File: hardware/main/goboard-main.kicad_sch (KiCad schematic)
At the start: 15 parts, among them J1 USB_C_Receptacle_USB2.0, J2 Conn_02x05_Top_Bottom, J3 Conn_01x01, J4 Conn_01x05, SW11 SW_Push, SW30 SW_DP3T

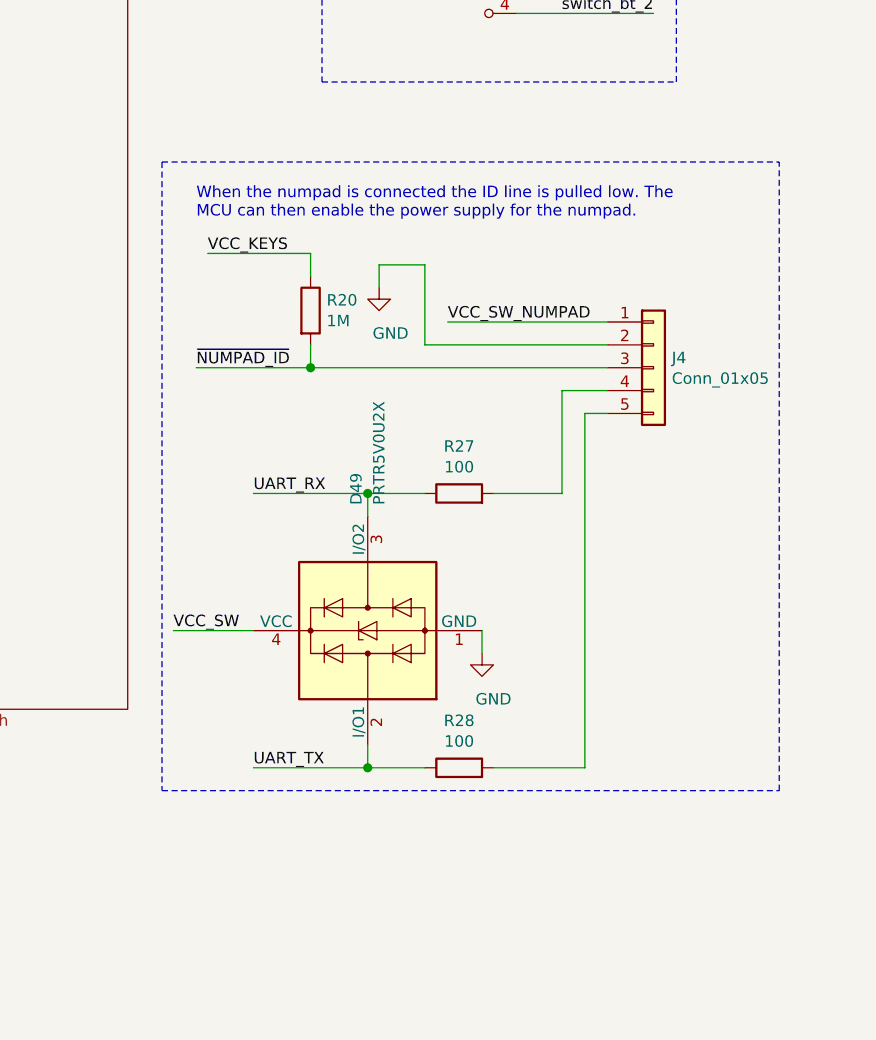
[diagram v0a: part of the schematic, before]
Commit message: WIP: Design of PCB
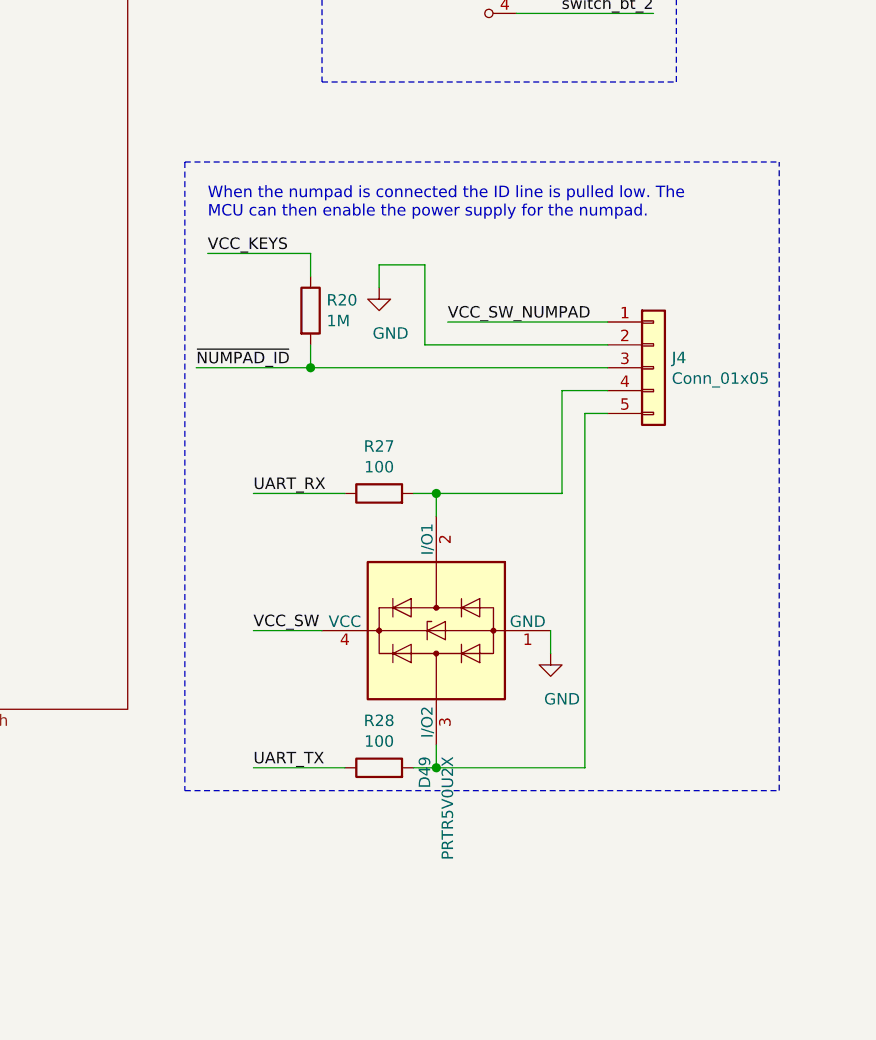
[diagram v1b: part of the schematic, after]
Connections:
- net UART_RX: no longer D49.3 (I/O2)
- net UART_TX: no longer D49.2 (I/O1)
- net at J4.4 (Pin_4), R27.2: now also D49.2 (I/O1)
- net at J4.5 (Pin_5), R28.2: now also D49.3 (I/O2)
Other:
- moved on the sheet: D49, R27, R28
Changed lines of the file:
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@@
   (junction (at 80.01 91.44) (diameter 1.016) (color 0 0 0 0))
   (junction (at 232.41 109.22) (diameter 1.016) (color 0 0 0 0))
-  (junction (at 238.76 123.19) (diameter 1.016) (color 0 0 0 0))
-  (junction (at 238.76 153.67) (diameter 1.016) (color 0 0 0 0))
+  (junction (at 246.38 123.19) (diameter 1.016) (color 0 0 0 0))
+  (junction (at 246.38 153.67) (diameter 1.016) (color 0 0 0 0))
   (no_connect (at 33.02 165.1))
   (no_connect (at 33.02 170.18))
@@
     (stroke (width 0) (type solid) (color 0 0 0 0))
   )
-  (wire (pts (xy 217.17 138.43) (xy 226.06 138.43))
-    (stroke (width 0) (type solid) (color 0 0 0 0))
-  )
   (wire (pts (xy 219.71 109.22) (xy 232.41 109.22))
     (stroke (width 0) (type solid) (color 0 0 0 0))
@@
     (stroke (width 0) (type solid) (color 0 0 0 0))
   )
-  (wire (pts (xy 226.06 123.19) (xy 238.76 123.19))
-    (stroke (width 0) (type solid) (color 0 0 0 0))
-  )
-  (wire (pts (xy 226.06 153.67) (xy 238.76 153.67))
+  (wire (pts (xy 226.06 123.19) (xy 236.22 123.19))
+    (stroke (width 0) (type solid) (color 0 0 0 0))
+  )
+  (wire (pts (xy 226.06 138.43) (xy 233.68 138.43))
+    (stroke (width 0) (type solid) (color 0 0 0 0))
+  )
+  (wire (pts (xy 226.06 153.67) (xy 236.22 153.67))
     (stroke (width 0) (type solid) (color 0 0 0 0))
   )
@@
     (stroke (width 0) (type solid) (color 0 0 0 0))
   )
-  (wire (pts (xy 238.76 123.19) (xy 238.76 125.73))
-    (stroke (width 0) (type solid) (color 0 0 0 0))
-  )
-  (wire (pts (xy 238.76 123.19) (xy 245.11 123.19))
-    (stroke (width 0) (type solid) (color 0 0 0 0))
-  )
-  (wire (pts (xy 238.76 151.13) (xy 238.76 153.67))
-    (stroke (width 0) (type solid) (color 0 0 0 0))
-  )
-  (wire (pts (xy 238.76 153.67) (xy 245.11 153.67))
-    (stroke (width 0) (type solid) (color 0 0 0 0))
-  )
   (wire (pts (xy 240.03 97.79) (xy 240.03 100.33))
     (stroke (width 0) (type solid) (color 0 0 0 0))
@@
     (stroke (width 0) (type solid) (color 0 0 0 0))
   )
+  (wire (pts (xy 243.84 123.19) (xy 246.38 123.19))
+    (stroke (width 0) (type solid) (color 0 0 0 0))
+  )
+  (wire (pts (xy 243.84 153.67) (xy 246.38 153.67))
+    (stroke (width 0) (type solid) (color 0 0 0 0))
+  )
   (wire (pts (xy 245.11 97.79) (xy 245.11 106.68))
     (stroke (width 0) (type solid) (color 0 0 0 0))
@@
     (stroke (width 0) (type solid) (color 0 0 0 0))
   )
+  (wire (pts (xy 246.38 123.19) (xy 246.38 125.73))
+    (stroke (width 0) (type solid) (color 0 0 0 0))
+  )
+  (wire (pts (xy 246.38 123.19) (xy 260.35 123.19))
+    (stroke (width 0) (type solid) (color 0 0 0 0))
+  )
+  (wire (pts (xy 246.38 151.13) (xy 246.38 153.67))
+    (stroke (width 0) (type solid) (color 0 0 0 0))
+  )
+  (wire (pts (xy 246.38 153.67) (xy 262.89 153.67))
+    (stroke (width 0) (type solid) (color 0 0 0 0))
+  )
   (wire (pts (xy 247.65 104.14) (xy 265.43 104.14))
     (stroke (width 0) (type solid) (color 0 0 0 0))
   )
-  (wire (pts (xy 251.46 138.43) (xy 251.46 140.97))
-    (stroke (width 0) (type solid) (color 0 0 0 0))
-  )
-  (wire (pts (xy 252.73 123.19) (xy 260.35 123.19))
-    (stroke (width 0) (type solid) (color 0 0 0 0))
-  )
   (wire (pts (xy 255.27 67.31) (xy 270.51 67.31))
     (stroke (width 0) (type solid) (color 0 0 0 0))
@@
     (stroke (width 0) (type solid) (color 0 0 0 0))
   )
+  (wire (pts (xy 259.08 138.43) (xy 259.08 140.97))
+    (stroke (width 0) (type solid) (color 0 0 0 0))
+  )
   (wire (pts (xy 260.35 111.76) (xy 265.43 111.76))
     (stroke (width 0) (type solid) (color 0 0 0 0))
@@
     (stroke (width 0) (type solid) (color 0 0 0 0))
   )
-  (wire (pts (xy 262.89 153.67) (xy 252.73 153.67))
-    (stroke (width 0) (type solid) (color 0 0 0 0))
-  )
   (wire (pts (xy 265.43 114.3) (xy 262.89 114.3))
     (stroke (width 0) (type solid) (color 0 0 0 0))
   )
-  (polyline (pts (xy 215.9 86.36) (xy 215.9 156.21))
+  (polyline (pts (xy 218.44 86.36) (xy 218.44 156.21))
     (stroke (width 0) (type dash) (color 0 0 0 0))
   )
-  (polyline (pts (xy 215.9 86.36) (xy 284.48 86.36))
+  (polyline (pts (xy 218.44 86.36) (xy 284.48 86.36))
     (stroke (width 0) (type dash) (color 0 0 0 0))
   )
-  (polyline (pts (xy 215.9 156.21) (xy 284.48 156.21))
+  (polyline (pts (xy 218.44 156.21) (xy 284.48 156.21))
     (stroke (width 0) (type dash) (color 0 0 0 0))
   )
@@
   )
   (text "When the numpad is connected the ID line is pulled low. The\nMCU can then enable the power supply for the numpad."
-    (at 219.71 92.71 0)
+    (at 220.98 92.71 0)
     (effects (font (size 1.27 1.27)) (justify left bottom))
   )
@@
     (effects (font (size 1.27 1.27)) (justify right bottom))
   )
-  (label "VCC_SW" (at 217.17 138.43 0)
-    (effects (font (size 1.27 1.27)) (justify left bottom))
-  )
   (label "~NUMPAD_ID" (at 219.71 109.22 0)
     (effects (font (size 1.27 1.27)) (justify left bottom))
@@
   )
   (label "UART_RX" (at 226.06 123.19 0)
+    (effects (font (size 1.27 1.27)) (justify left bottom))
+  )
+  (label "VCC_SW" (at 226.06 138.43 0)
     (effects (font (size 1.27 1.27)) (justify left bottom))
   )
@@
     )
   )
-  (symbol (lib_id "power:GND") (at 251.46 140.97 0) (unit 1)
-    (in_bom yes) (on_board yes)
-    (property "Reference" "#PWR0123" (id 0) (at 251.46 147.32 0)
-      (effects (font (size 1.27 1.27)) hide)
-    )
-    (property "Value" "GND" (id 1) (at 252.73 146.05 0))
-    (property "Footprint" "" (id 2) (at 251.46 140.97 0)
-      (effects (font (size 1.27 1.27)) hide)
-    )
-    (property "Datasheet" "" (id 3) (at 251.46 140.97 0)
+  (symbol (lib_id "power:GND") (at 259.08 140.97 0) (unit 1)
+    (in_bom yes) (on_board yes)
+    (property "Reference" "#PWR0123" (id 0) (at 259.08 147.32 0)
+      (effects (font (size 1.27 1.27)) hide)
+    )
+    (property "Value" "GND" (id 1) (at 260.35 146.05 0))
+    (property "Footprint" "" (id 2) (at 259.08 140.97 0)
+      (effects (font (size 1.27 1.27)) hide)
+    )
+    (property "Datasheet" "" (id 3) (at 259.08 140.97 0)
       (effects (font (size 1.27 1.27)) hide)
     )
@@
     )
   )
-  (symbol (lib_id "Device:R") (at 248.92 123.19 90) (unit 1)
-    (in_bom yes) (on_board yes)
-    (property "Reference" "R27" (id 0) (at 248.92 117.9638 90))
-    (property "Value" "100" (id 1) (at 248.92 120.2625 90))
-    (property "Footprint" "Resistor_SMD:R_0603_1608Metric_Pad0.98x0.95mm_HandSolder" (id 2) (at 248.92 124.968 90)
-      (effects (font (size 1.27 1.27)) hide)
-    )
-    (property "Datasheet" "~" (id 3) (at 248.92 123.19 0)
-      (effects (font (size 1.27 1.27)) hide)
-    )
-  )
-  (symbol (lib_id "Device:R") (at 248.92 153.67 90) (unit 1)
-    (in_bom yes) (on_board yes)
-    (property "Reference" "R28" (id 0) (at 248.92 148.4438 90))
-    (property "Value" "100" (id 1) (at 248.92 150.7425 90))
-    (property "Footprint" "Resistor_SMD:R_0603_1608Metric_Pad0.98x0.95mm_HandSolder" (id 2) (at 248.92 155.448 90)
-      (effects (font (size 1.27 1.27)) hide)
-    )
-    (property "Datasheet" "~" (id 3) (at 248.92 153.67 0)
+  (symbol (lib_id "Device:R") (at 240.03 123.19 90) (unit 1)
+    (in_bom yes) (on_board yes)
+    (property "Reference" "R27" (id 0) (at 240.03 117.9638 90))
+    (property "Value" "100" (id 1) (at 240.03 120.2625 90))
+    (property "Footprint" "Resistor_SMD:R_0603_1608Metric_Pad0.98x0.95mm_HandSolder" (id 2) (at 240.03 124.968 90)
+      (effects (font (size 1.27 1.27)) hide)
+    )
+    (property "Datasheet" "~" (id 3) (at 240.03 123.19 0)
+      (effects (font (size 1.27 1.27)) hide)
+    )
+  )
+  (symbol (lib_id "Device:R") (at 240.03 153.67 90) (unit 1)
+    (in_bom yes) (on_board yes)
+    (property "Reference" "R28" (id 0) (at 240.03 148.4438 90))
+    (property "Value" "100" (id 1) (at 240.03 150.7425 90))
+    (property "Footprint" "Resistor_SMD:R_0603_1608Metric_Pad0.98x0.95mm_HandSolder" (id 2) (at 240.03 155.448 90)
+      (effects (font (size 1.27 1.27)) hide)
+    )
+    (property "Datasheet" "~" (id 3) (at 240.03 153.67 0)
       (effects (font (size 1.27 1.27)) hide)
     )
@@
     )
   )
-  (symbol (lib_id "Power_Protection:PRTR5V0U2X") (at 238.76 138.43 90) (unit 1)
-    (in_bom yes) (on_board yes)
-    (property "Reference" "D49" (id 0) (at 237.49 124.46 0)
-      (effects (font (size 1.27 1.27)) (justify left))
-    )
-    (property "Value" "PRTR5V0U2X" (id 1) (at 240.03 124.46 0)
-      (effects (font (size 1.27 1.27)) (justify left))
-    )
-    (property "Footprint" "Package_TO_SOT_SMD:SOT-143" (id 2) (at 238.76 136.906 0)
-      (effects (font (size 1.27 1.27)) hide)
-    )
-    (property "Datasheet" "https://assets.nexperia.com/documents/data-sheet/PRTR5V0U2X.pdf" (id 3) (at 238.76 136.906 0)
-      (effects (font (size 1.27 1.27)) hide)
-    )
-    (property "Mouser" " 771-PRTR5V0U2X-T/R " (id 4) (at 238.76 138.43 0)
-      (effects (font (size 1.27 1.27)) hide)
-    )
-    (property "Part Name" "PRTR5V0U2X,215" (id 5) (at 238.76 138.43 0)
-      (effects (font (size 1.27 1.27)) hide)
-    )
+  (symbol (lib_id "Power_Protection:PRTR5V0U2X") (at 246.38 138.43 90) (mirror x) (unit 1)
+    (in_bom yes) (on_board yes)
+    (property "Reference" "D49" (id 0) (at 245.11 152.4 0)
+      (effects (font (size 1.27 1.27)) (justify left))
+    )
+    (property "Value" "PRTR5V0U2X" (id 1) (at 247.65 152.4 0)
+      (effects (font (size 1.27 1.27)) (justify left))
+    )
+    (property "Footprint" "Package_TO_SOT_SMD:SOT-143" (id 2) (at 246.38 139.954 0)
+      (effects (font (size 1.27 1.27)) hide)
+    )
+    (property "Datasheet" "https://assets.nexperia.com/documents/data-sheet/PRTR5V0U2X.pdf" (id 3) (at 246.38 139.954 0)
+      (effects (font (size 1.27 1.27)) hide)
+    )
+    (property "Mouser" " 771-PRTR5V0U2X-T/R " (id 4) (at 246.38 138.43 0)
+      (effects (font (size 1.27 1.27)) hide)
+    )
+    (property "Part Name" "PRTR5V0U2X,215" (id 5) (at 246.38 138.43 0)
+      (effects (font (size 1.27 1.27)) hide)
+    )
